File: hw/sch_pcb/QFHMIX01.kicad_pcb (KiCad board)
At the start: 2 copper layers, 90.9 x 90.9 mm, 205 parts, among them J1 HEADER_1x08, J2 +9V, M1 HOLE, M2 HOLE, M3 HOLE, M4 HOLE, M5 HOLE, M6 HOLE, M7 HOLE, M8 HOLE, U1 NCP1117ST33, U11 TPS563249, U12 Si53322, U2 AD8343, U3 AD8343, U5 LT6604-10, U6 MPGA-105+, U7 MPGA-105+, U8 MGVA-63+, U9 MGVA-63+

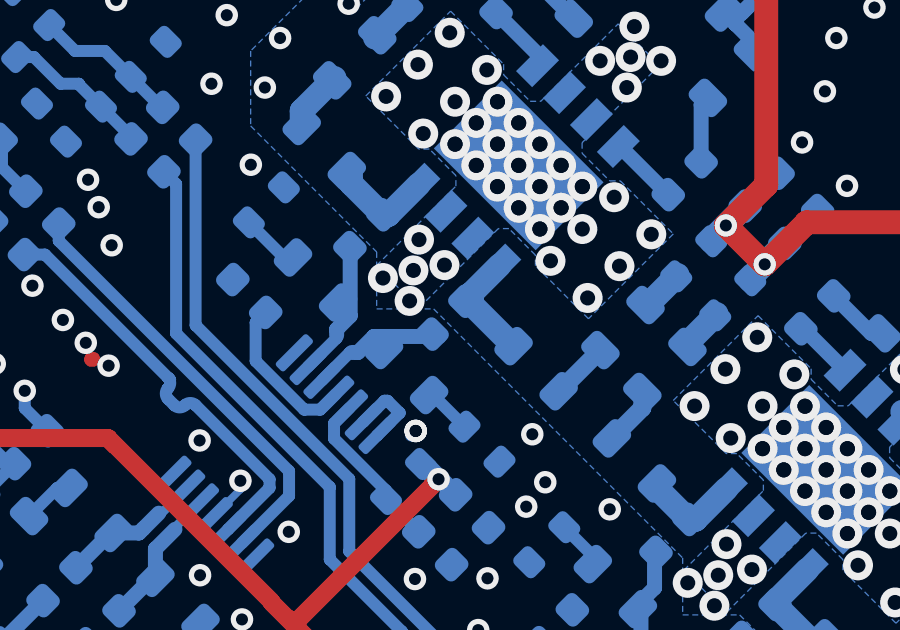
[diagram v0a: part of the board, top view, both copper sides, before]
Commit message: Edit PCB
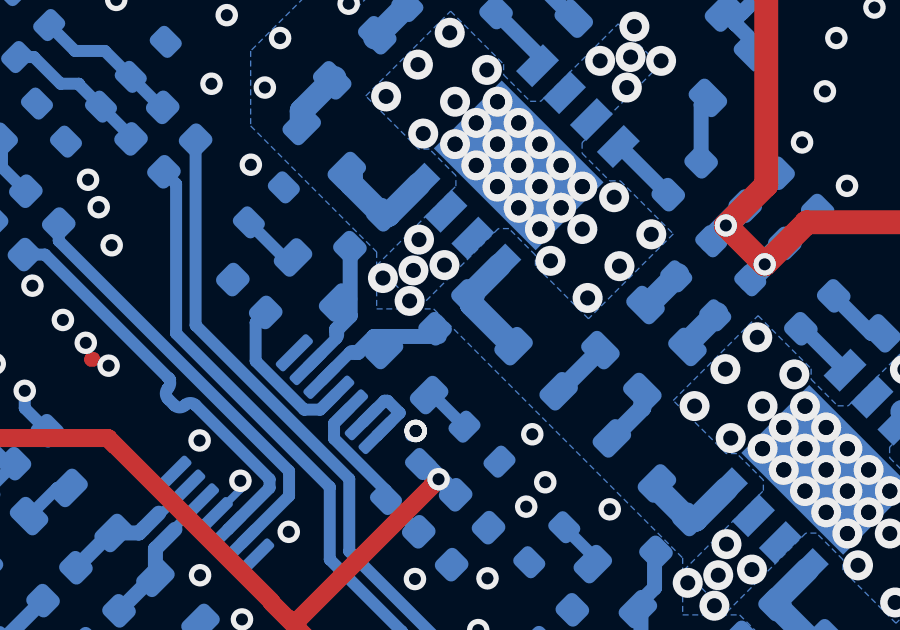
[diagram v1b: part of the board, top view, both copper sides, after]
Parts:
- moved C36 0.20 mm to (144.5, 87.9)
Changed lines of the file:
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@@
-(kicad_pcb (version 20210606) (generator pcbnew)
+(kicad_pcb (version 20210228) (generator pcbnew)
   (general
     (thickness 1.6)
@@
   )
   (footprint "Capacitor_SMD:C_0603_1608Metric" (layer "B.Cu")
-    (at 144.4244 88.0618 -135)
-    (descr "Capacitor SMD 0603 (1608 Metric), square (rectangular) end terminal, IPC_7351 nominal, (Body size source: IPC-SM-782 page 76, https://www.pcb-3d.com/wordpress/wp-content/uploads/ipc-sm-782a_amendment_1_and_2.pdf), generated with kicad-footprint-generator")
-    (tags "capacitor")
+    (at 144.526 87.884 -135)
+    (descr "Capacitor SMD 0603 (1608 Metric), square (rectangular) end terminal, IPC_7351 nominal, (Body size source: IPC-SM-782 page 76, https://www.pcb-3d.com/wordpress/wp-content/uploads/ipc-sm-782a_amendment_1_and_2.pdf), generated with kicad-footprint-generator")
+    (tags "capacitor")
